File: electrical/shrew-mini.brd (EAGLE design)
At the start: 14 x 11 mm, 18 parts, among them IC1 Vreg +3V3, U1 DRV8231DSGR, U2 DRV8231DSGR, X1 PIN-1X-BIG, X2 PIN-1X-BIG, X3 PIN-1X-BIG, X4 PIN-1X-BIG, X5 PIN-1X-1.5MMSQ, X6 PIN-1X-MED

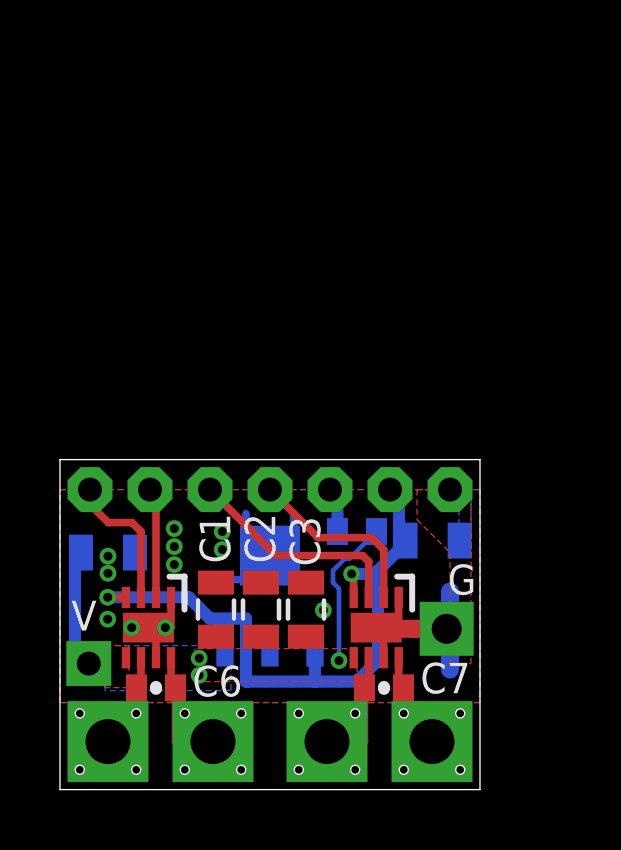
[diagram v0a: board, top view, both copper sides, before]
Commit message: up-rev
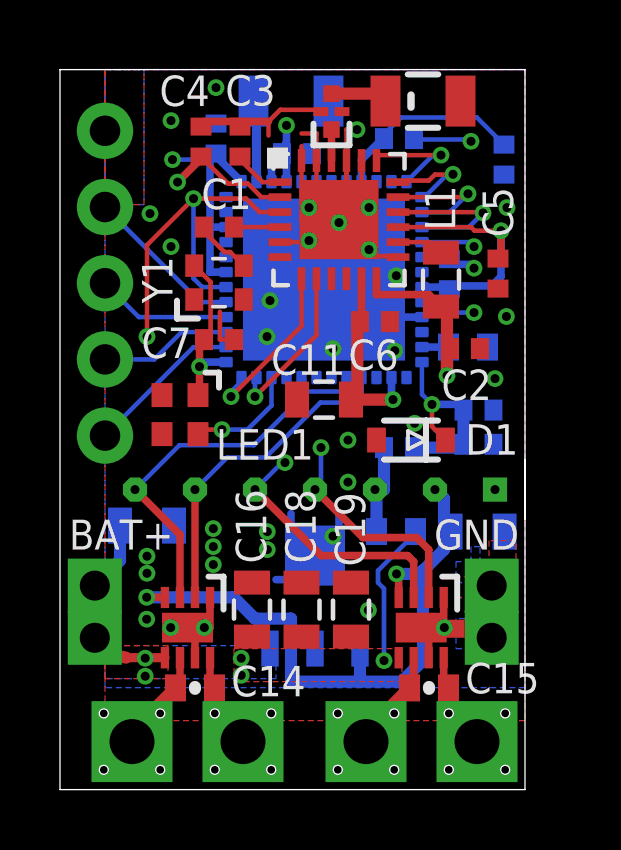
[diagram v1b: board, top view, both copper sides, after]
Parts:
- added ANT1, ANT2: 74889302450, shrew-common:ANTENNA-CHIP2
- added C10, C8, C9: 100n, shrew-common:0402-REV
- added C11: 10uF 25V, shrew-common:0805
- added C12: DNP, shrew-common:0402-CAP
- added C13, C17: 470n, shrew-common:0402-REV
- added C14, C15: (no value), shrew-common:0402-CAP
- added C16, C18, C19, C20, C21: (no value), shrew-common:0805
- added D1: 3V6, shrew-common:SOD-323
- added EDGE1: (no value), shrew-common:1X05
- added FL1: 2450FM07D0034T, shrew-core:FIL_2450FM07D0034T
- added L1: 15u, shrew-common:0805
- added LED1: SK6812-EC20, shrew-core:SK6812-EC20
- added R2, R3: 10K, shrew-common:0402-REV
- added R4: (no value), shrew-common:0402-RES
- added U3, U4: DRV8231DSGR, shrew-core:WSON8_DRV8231_TEX
- added X7, X8: PIN-1X-MED, shrew-core:PAD-1X-MED
- added Y1: 52MHz TCXO, shrew-common:OSC_TG2016SMN_50.0000M-ECGNNMB
- C1: value (none) -> 1n; device shrew-common:0805 -> shrew-common:0402-REV
- C2: value (none) -> 470n; device shrew-common:0805 -> shrew-common:0402-REV
- C3, C4: value (none) -> 10n; device shrew-common:0805 -> shrew-common:0402-REV
- C5: value (none) -> 100n; device shrew-common:0805 -> shrew-common:0402-REV
- C6, C7: value (none) -> 100n; device shrew-common:0402-CAP -> shrew-common:0402-REV
- JP1: device shrew-common:1X07-2MM-TH -> shrew-common:1X07-2MM-TH-TINY
- R1: value (none) -> 10K; device shrew-common:0402-RES -> shrew-common:0402-REV
- U1: value DRV8231DSGR -> ESP32-PICO-D4; device shrew-core:WSON8_DRV8231_TEX -> shrew-core:PQFN50P700X700X104-49N
- U2: value DRV8231DSGR -> SX1280IMLTRT; device shrew-core:WSON8_DRV8231_TEX -> shrew-core:QFN24_4X4_SEM
- X5: value PIN-1X-1.5MMSQ -> PIN-1X-MED; device shrew-core:PAD-1X-1.5MMSQ -> shrew-core:PAD-1X-MED
- moved C3 15.8 mm to (6.00, 21.6), turned to 270 degrees
- moved U2 15.0 mm to (9.30, 19.0), turned to 0 degrees
- moved C6 14.2 mm to (10.5, 15.6)
- moved C4 14.0 mm to (4.70, 21.6), flipped to the top, turned to 270 degrees
- moved R1 13.2 mm to (11.3, 21.7)
- moved C7 12.8 mm to (5.30, 15.0)
- moved C1 12.8 mm to (5.30, 18.8), turned to 0 degrees
- moved U1 11.7 mm to (8.80, 17.0), flipped to the bottom
- moved C2 11.0 mm to (13.5, 14.7), turned to 180 degrees
- moved C5 9.16 mm to (14.6, 17.2), flipped to the top, turned to 90 degrees
- moved X6 1.53 mm to (14.4, 5.06)
- moved IC1 1.50 mm to (8.50, 6.50)
- moved JP1 1.50 mm to (8.50, 10.0), turned to 0 degrees
- moved X4 1.50 mm to (13.9, 1.60)
- moved X3 1.30 mm to (10.2, 1.60)
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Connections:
- new net AUX1: EDGE1.1, U1.38
- new net AUX2: EDGE1.2, U1.39
- new net BATT-ADC: C17.1, D1.1, R2.2, R3.1, U1.24
- new net ESP-BOOT: C12.2, U1.23
- new net ESP-EN: C13.2, R1.1, U1.9
- new net N$1: ANT1.FEED, U1.2
- new net N$11: C3.2, U2.1
- new net N$2: C1.1, Y1.3
- new net N$3: C1.2, U2.4
- new net N$5: U1.17
- new net N$6: FL1.1, U2.22
- new net N$7: ANT2.FEED, FL1.3
- new net N$8: U1.22
- new net N$9: L1.2, U2.14
- new net RADIO-BUSY: U1.36, U2.7
- new net RADIO-CS: U1.12, U2.19
- new net RADIO-DIO: U1.35, U2.8
- new net RADIO-RST: U1.42, U2.3
- new net RADIO-VDD: C2.2, C4.2, L1.1, U2.12, U2.2
- new net RGBLED: LED1.4, U1.34
- new net SPI-MISO: U1.15, U2.16
- new net SPI-MOSI: U1.14, U2.17
- new net SPI-SCK: U1.13, U2.18
- new net U0RXD: EDGE1.3, U1.40
- new net U0TXD: EDGE1.4, U1.41
- net +24V: now also C16.1, C18.1, C19.1, C20.1, R4.2, U3.5, U4.5, X5.1, X7.1; no longer C1.1, C2.1, C3.1, C4.1, R1.2, U1.5, U2.5, X5.P$1
- net 3.3V: now also C10.1, C11.1, C21.1, C5.2, C6.2, C7.2, C8.1, C9.1, LED1.1, R1.2, U1.1, U1.19, U1.26, U1.3, U1.37, U1.43, U1.46, U2.11, U2.15, U3.4, U4.4, Y1.4; no longer C5.1, U2.4
- net GND: now also C10.2, C11.2, C12.1, C13.1, C16.2, C17.2, C18.2, C19.2, C2.1, C20.2, C21.2, C3.1, C4.1, C5.1, C6.1, C7.1, C8.2, C9.2, D1.2, EDGE1.5, FL1.2, FL1.4, LED1.3, R2.1, U1.21, U1.49, U2.13, U2.20, U2.21, U2.23, U2.24, U2.25, U2.5, U3.1, U3.7, U3.9, U4.1, U4.7, U4.9, X6.1, X8.1, Y1.2; no longer C1.2, C2.2, C3.2, C4.2, C5.2, U1.1, U1.7, U1.9, U2.1, U2.7, U2.9, X6.P$1
- net MOTOR1: now also C15.2, U4.6; no longer C7.2, U1.6
- net MOTOR2: now also C15.1, U4.8; no longer C7.1, U1.8
- net MOTOR3: now also C14.2, U3.6; no longer C6.2, U2.6
- net MOTOR4: now also C14.1, U3.8; no longer C6.1, U2.8
- net SIG1: now also U1.20, U4.2; no longer U1.2
- net SIG2: now also U1.16, U4.3; no longer U1.3
- net SIG3: now also U1.28, U3.2; no longer U2.2
- net SIG4: now also U1.29, U3.3; no longer U2.3
- net V-ADC: now also R3.2, R4.1; no longer R1.1
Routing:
- net GND: track 16.9 -> 53.4 mm, vias 11 -> 35
- net 3.3V: track 21.7 -> 56.1 mm, vias 2 -> 8
- net RADIO-VDD: track 0.00 -> 22.8 mm, vias 0 -> 2
- net SIG2: track 7.48 -> 22.0 mm, vias 0 -> 2
- net RADIO-RST: track 0.00 -> 12.2 mm, vias 0 -> 2
- net SIG1: track 6.22 -> 17.2 mm, vias 0 -> 2
- net SIG4: track 4.76 -> 13.0 mm
- net SIG3: track 3.68 -> 11.0 mm
- net BATT-ADC: track 0.00 -> 6.98 mm, vias 0 -> 1
- net ESP-EN: track 0.00 -> 6.52 mm
- net RADIO-BUSY: track 0.00 -> 5.77 mm, vias 0 -> 1
- net RADIO-DIO: track 0.00 -> 5.47 mm, vias 0 -> 1
- net U0TXD: track 0.00 -> 5.35 mm
- net AUX1: track 0.00 -> 5.26 mm
- net SPI-MISO: track 0.00 -> 5.07 mm, vias 0 -> 1
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- added copper zone on layer 15, net +24V
- added copper zone on layer 15, net 3.3V
- added copper zone on layer 2, net GND
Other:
- board size 14 x 11 mm -> 15.5 x 24 mm
- board text added: "1"
- board text added: "19"
- board text added: "22"
- board text added: "3"
- board text added: "BAT+"
- board text added: "GND"
- board text added: "P1"
- board text added: "P2"
- board text added: "RX"
- board text added: "TX"
- board text removed: "V"
